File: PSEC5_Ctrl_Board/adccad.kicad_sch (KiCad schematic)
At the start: 2 parts, among them U13 LTC2600CGN_PBF, U14 LTC2600CGN_PBF

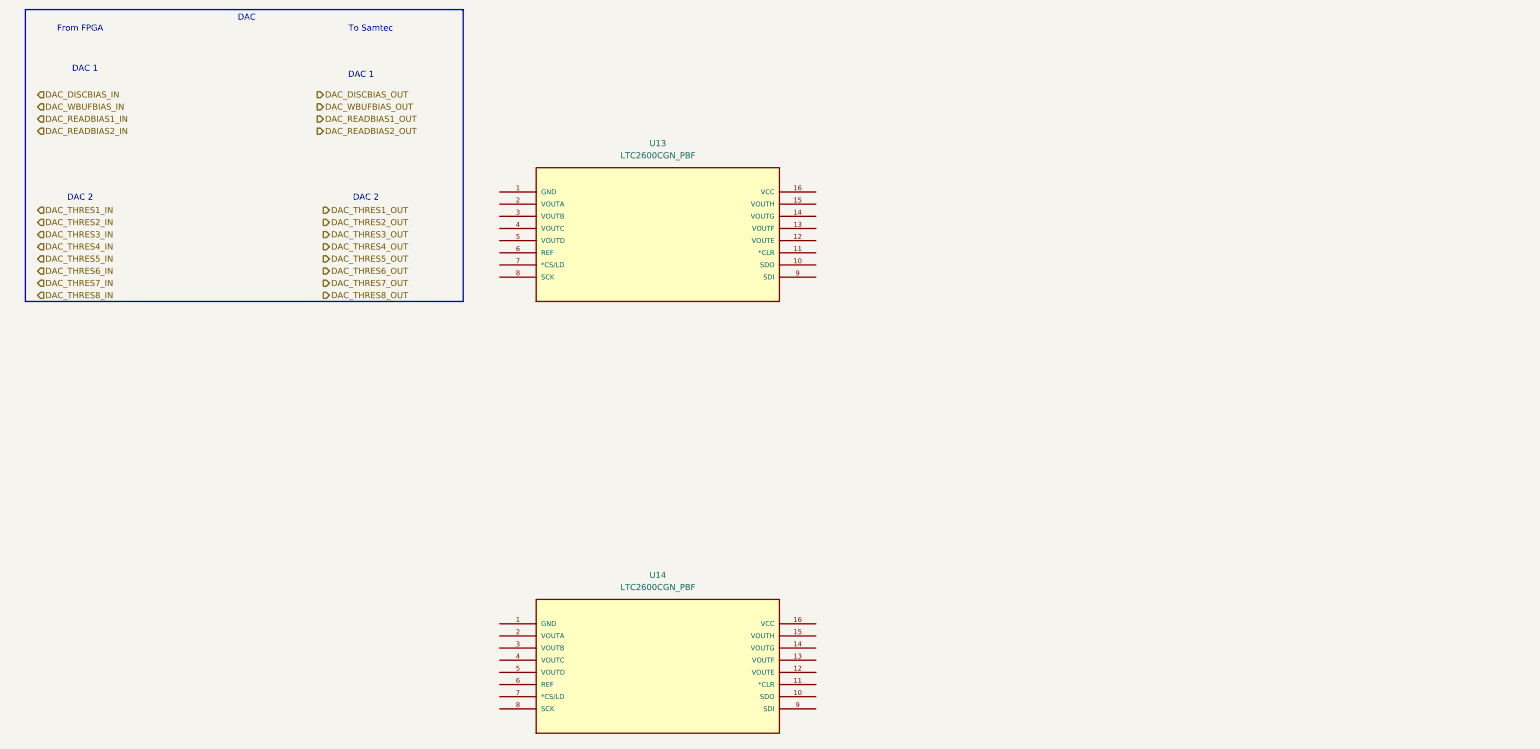
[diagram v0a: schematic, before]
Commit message: Large Updates, Touching up before further aproval
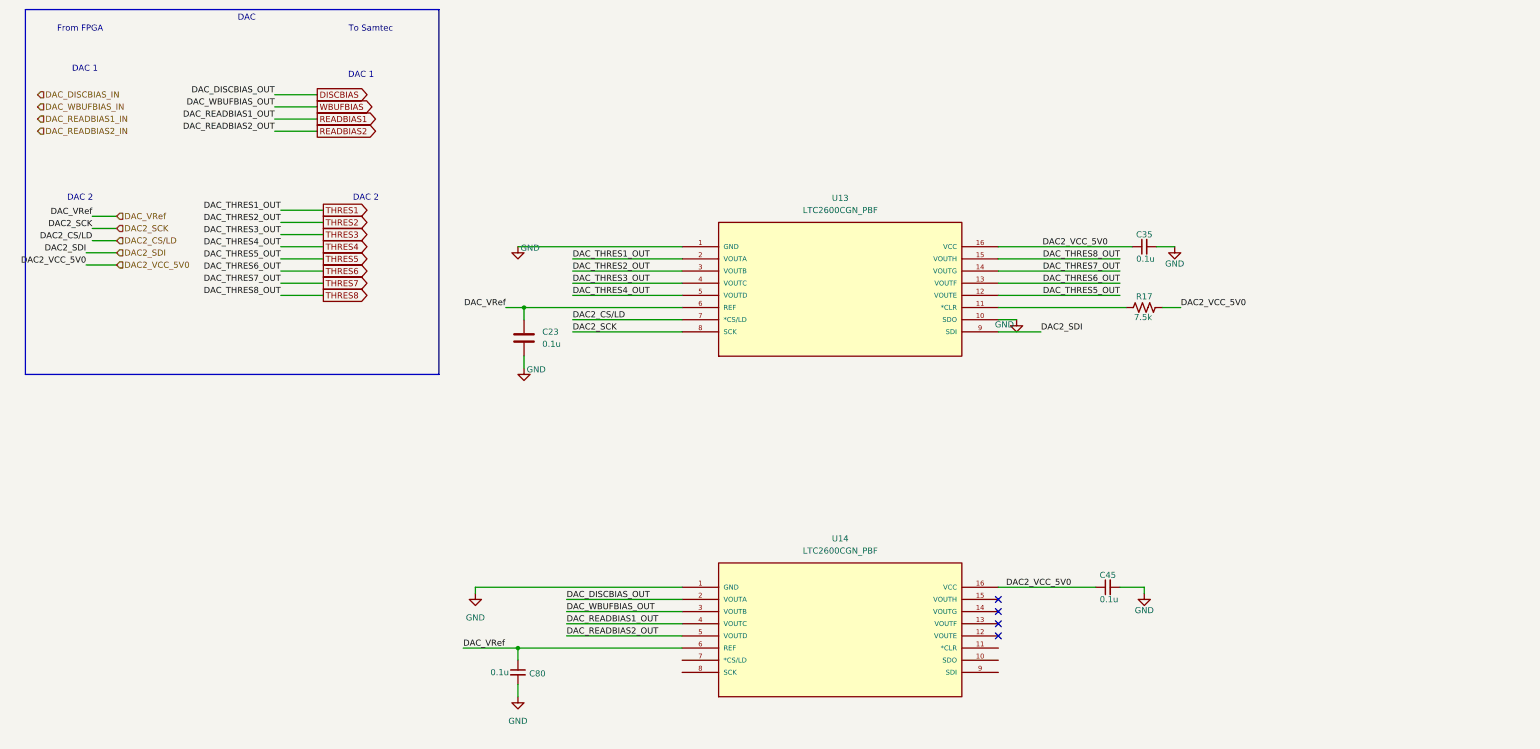
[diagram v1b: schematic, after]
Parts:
- added C23: 0.1u, symbol Device:C
- added C35, C45, C80: 0.1u, Capacitor_SMD:C_0201_0603Metric, symbol Device:C_Small
- added R17: 7.5k, symbol Device:R_US
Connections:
- net GND: now reaches U14.1 (GND)
- net GND: now also U13.1 (GND), U13.10 (SDO), C23.2, C35.2, C45.2, C80.2
- net DAC2_VCC_5V0: now reaches U14.16 (VCC)
- net DAC2_VCC_5V0: now also U13.16 (VCC), C35.1, C45.1, R17.2
- net DISCBIAS: now reaches U14.2 (VOUTA)
- net WBUFBIAS: now reaches U14.3 (VOUTB)
- net READBIAS1: now reaches U14.4 (VOUTC)
- net READBIAS2: now reaches U14.5 (VOUTD)
- net DAC_VRef: now reaches U14.6 (REF)
- net DAC_VRef: now also U13.6 (REF), C23.1, C80.1
- net at U13.11 (*CLR): now also R17.1
- net THRES5: now reaches U13.12 (VOUTE)
- net THRES6: now reaches U13.13 (VOUTF)
- net THRES7: now reaches U13.14 (VOUTG)
- net THRES8: now reaches U13.15 (VOUTH)
- net THRES1: now reaches U13.2 (VOUTA)
- net THRES2: now reaches U13.3 (VOUTB)
- net THRES3: now reaches U13.4 (VOUTC)
- net THRES4: now reaches U13.5 (VOUTD)
- net DAC2_CS/LD: now reaches U13.7 (*CS/LD)
- net DAC2_SCK: now reaches U13.8 (SCK)
- net DAC2_SDI: now reaches U13.9 (SDI)
- no-connect marks 0 -> 4
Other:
- moved on the sheet: U13, U14

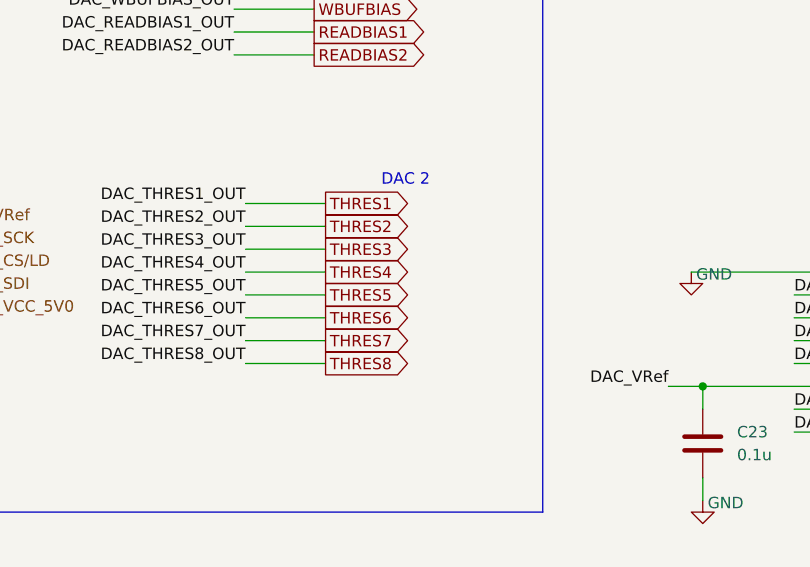
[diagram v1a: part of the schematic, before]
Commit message: minor changes
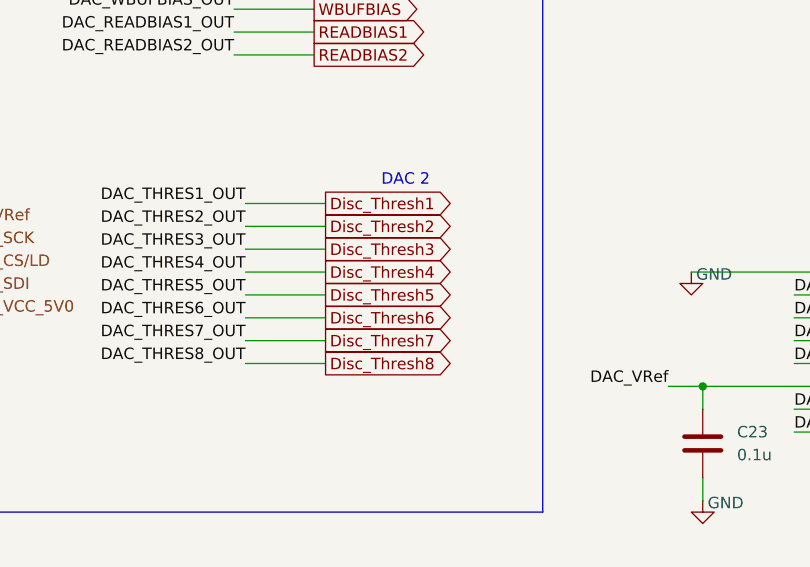
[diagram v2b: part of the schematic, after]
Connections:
- net THRES1 renamed Disc_Thresh1
- net THRES2 renamed Disc_Thresh2
- net THRES3 renamed Disc_Thresh3
- net THRES4 renamed Disc_Thresh4
- net THRES5 renamed Disc_Thresh5
- net THRES6 renamed Disc_Thresh6
- net THRES7 renamed Disc_Thresh7
- net THRES8 renamed Disc_Thresh8
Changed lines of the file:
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@@
 		)
 	)
-	(global_label "THRES1"
+	(global_label "Disc_Thresh1"
 		(shape output)
 		(at 74.93 54.61 0)
@@
 		)
 		(property "Intersheetrefs" "${INTERSHEET_REFS}"
-			(at 85.0513 54.61 0)
-			(effects
-				(font
-					(size 1.27 1.27)
-				)
-				(justify left)
-				(hide yes)
-			)
-		)
-	)
-	(global_label "THRES4"
+			(at 90.2523 54.61 0)
+			(effects
+				(font
+					(size 1.27 1.27)
+				)
+				(justify left)
+				(hide yes)
+			)
+		)
+	)
+	(global_label "Disc_Thresh4"
 		(shape output)
 		(at 74.93 62.23 0)
@@
 		)
 		(property "Intersheetrefs" "${INTERSHEET_REFS}"
-			(at 85.0513 62.23 0)
+			(at 90.2523 62.23 0)
 			(effects
 				(font
@@
 		)
 	)
-	(global_label "THRES8"
+	(global_label "Disc_Thresh8"
 		(shape output)
 		(at 74.93 72.39 0)
@@
 		)
 		(property "Intersheetrefs" "${INTERSHEET_REFS}"
-			(at 85.0513 72.39 0)
-			(effects
-				(font
-					(size 1.27 1.27)
-				)
-				(justify left)
-				(hide yes)
-			)
-		)
-	)
-	(global_label "THRES2"
+			(at 90.2523 72.39 0)
+			(effects
+				(font
+					(size 1.27 1.27)
+				)
+				(justify left)
+				(hide yes)
+			)
+		)
+	)
+	(global_label "Disc_Thresh2"
 		(shape output)
 		(at 74.93 57.15 0)
@@
 		)
 		(property "Intersheetrefs" "${INTERSHEET_REFS}"
-			(at 85.0513 57.15 0)
-			(effects
-				(font
-					(size 1.27 1.27)
-				)
-				(justify left)
-				(hide yes)
-			)
-		)
-	)
-	(global_label "THRES7"
+			(at 90.2523 57.15 0)
+			(effects
+				(font
+					(size 1.27 1.27)
+				)
+				(justify left)
+				(hide yes)
+			)
+		)
+	)
+	(global_label "Disc_Thresh7"
 		(shape output)
 		(at 74.93 69.85 0)
@@
 		)
 		(property "Intersheetrefs" "${INTERSHEET_REFS}"
-			(at 85.0513 69.85 0)
-			(effects
-				(font
-					(size 1.27 1.27)
-				)
-				(justify left)
-				(hide yes)
-			)
-		)
-	)
-	(global_label "THRES6"
+			(at 90.2523 69.85 0)
+			(effects
+				(font
+					(size 1.27 1.27)
+				)
+				(justify left)
+				(hide yes)
+			)
+		)
+	)
+	(global_label "Disc_Thresh6"
 		(shape output)
 		(at 74.93 67.31 0)
@@
 		)
 		(property "Intersheetrefs" "${INTERSHEET_REFS}"
-			(at 85.0513 67.31 0)
-			(effects
-				(font
-					(size 1.27 1.27)
-				)
-				(justify left)
-				(hide yes)
-			)
-		)
-	)
-	(global_label "THRES5"
+			(at 90.2523 67.31 0)
+			(effects
+				(font
+					(size 1.27 1.27)
+				)
+				(justify left)
+				(hide yes)
+			)
+		)
+	)
+	(global_label "Disc_Thresh5"
 		(shape output)
 		(at 74.93 64.77 0)
@@
 		)
 		(property "Intersheetrefs" "${INTERSHEET_REFS}"
-			(at 85.0513 64.77 0)
+			(at 90.2523 64.77 0)
 			(effects
 				(font
@@
 		)
 	)
-	(global_label "THRES3"
+	(global_label "Disc_Thresh3"
 		(shape output)
 		(at 74.93 59.69 0)
@@
 		)
 		(property "Intersheetrefs" "${INTERSHEET_REFS}"
-			(at 85.0513 59.69 0)
-			(effects
-				(font
+			(at 90.2523 59.69 0)
+			(effects
+				(font

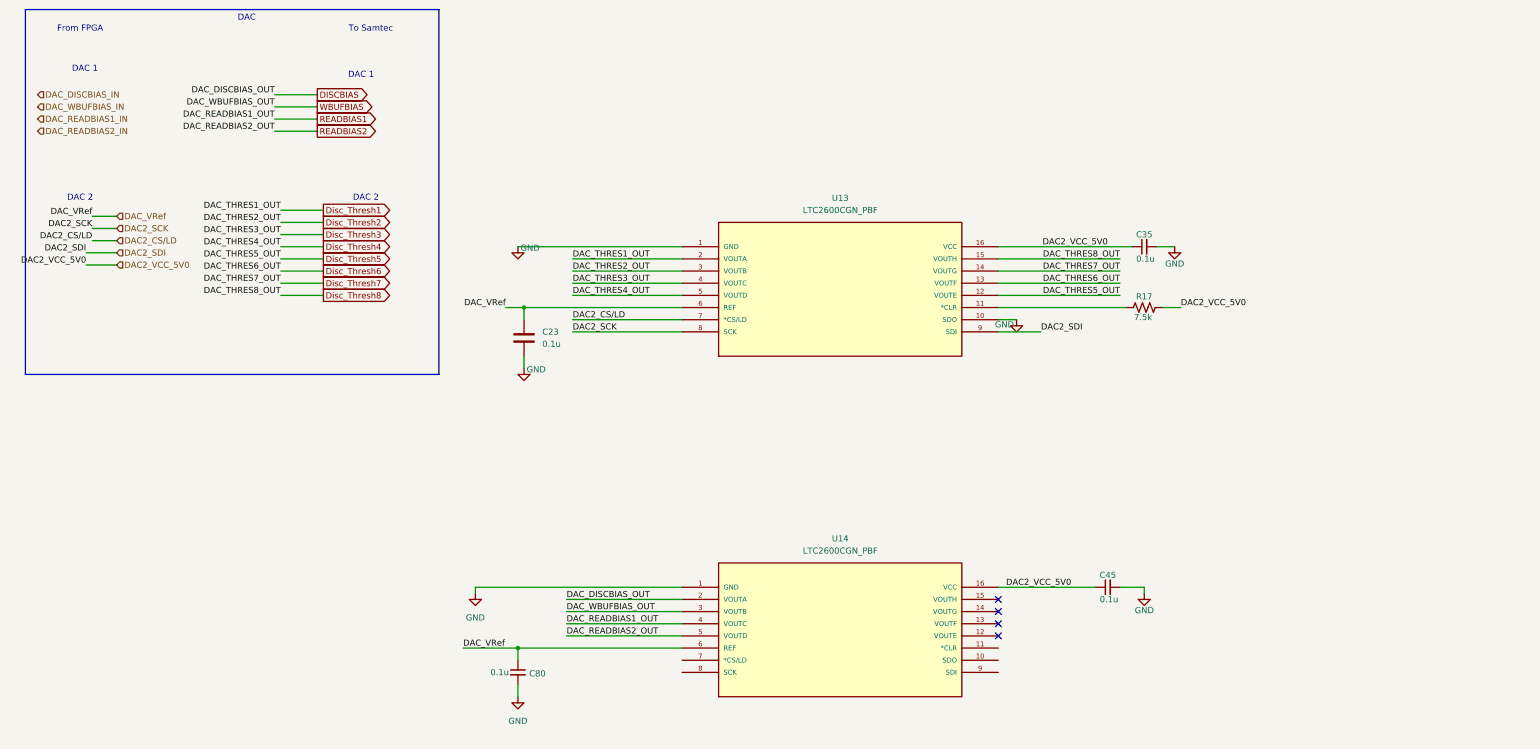
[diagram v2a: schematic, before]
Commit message: Schematic is "done" ;( (999+ ERC errors)
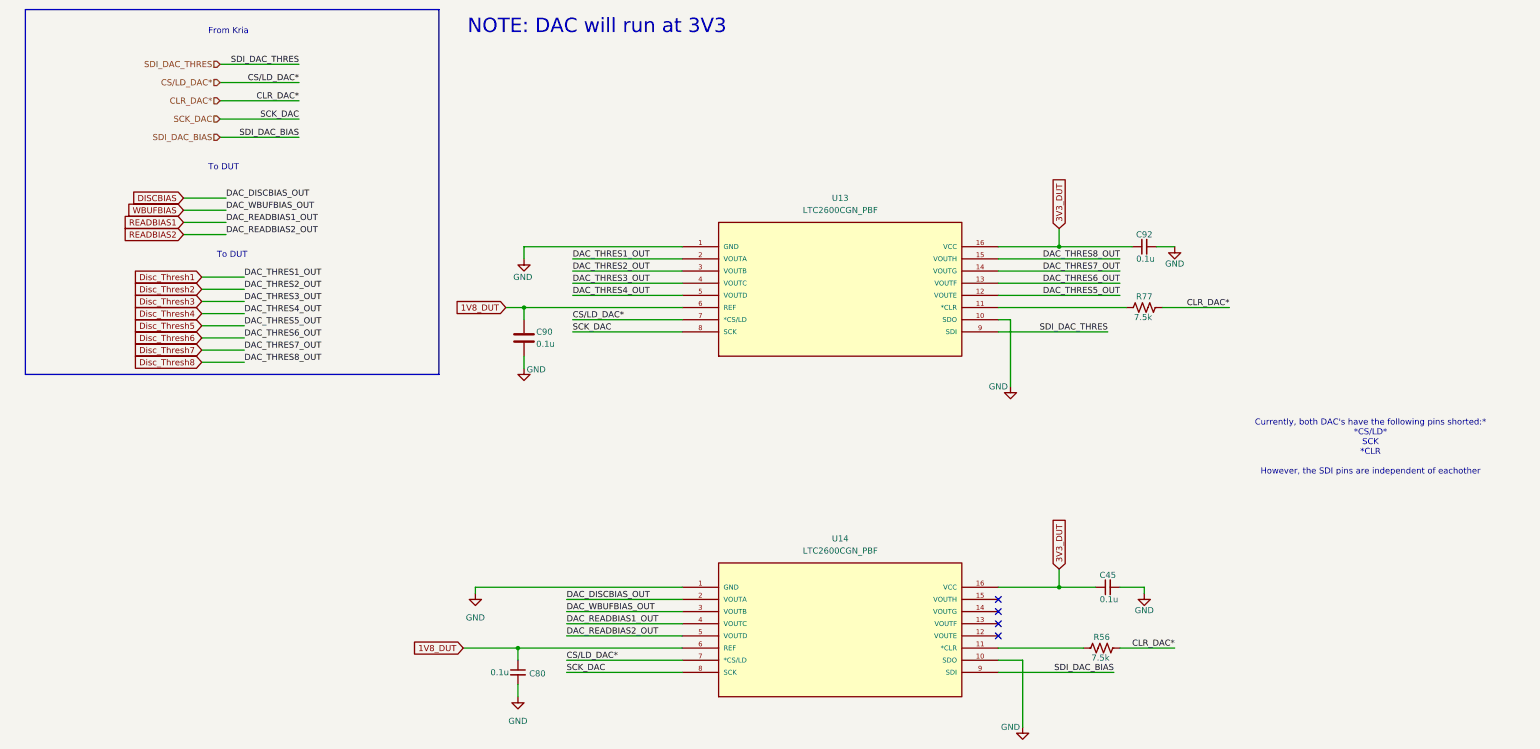
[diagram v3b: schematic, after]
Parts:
- added R56: 7.5k, Capacitor_SMD:C_0603_1608Metric, symbol Device:R_US
- C90: renamed from C23; footprint (none) -> Capacitor_SMD:C_0603_1608Metric
- R77: renamed from R17; footprint (none) -> Capacitor_SMD:C_0603_1608Metric
- renumbered C35 to C92
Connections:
- net DAC2_CS/LD is gone; now on net CS/LD_DAC*: U13.7 (*CS/LD)
- net DAC2_SCK is gone; now on net SCK_DAC: U13.8 (SCK)
- net GND: now also U14.10 (SDO)
- net at U14.11 (*CLR): now also R56.1
- net CS/LD_DAC*: now reaches U14.7 (*CS/LD)
- net SCK_DAC: now reaches U14.8 (SCK)
- net SDI_DAC_BIAS: now reaches U14.9 (SDI)
- net DAC2_SDI renamed SDI_DAC_THRES
- net DAC2_VCC_5V0 renamed 3V3_DUT
- net 3V3_DUT: no longer R77.2
- net DAC_VRef renamed 1V8_DUT
- new net CLR_DAC*: R56.2, R77.2
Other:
- note added: "Currently, both DAC's have the following pins shorted:* *CS/LD* SCK *CLR However, the SDI pins are independent of eachother"
- note added: "From Kria"
- note added: "NOTE: DAC will run at 3V3"
- note added: "To DUT"
- note removed: "DAC"
- note removed: "DAC 1"
- note removed: "DAC 2"
- note removed: "From FPGA"
- note removed: "To Samtec"
